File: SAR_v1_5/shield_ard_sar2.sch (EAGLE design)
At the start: 16 parts

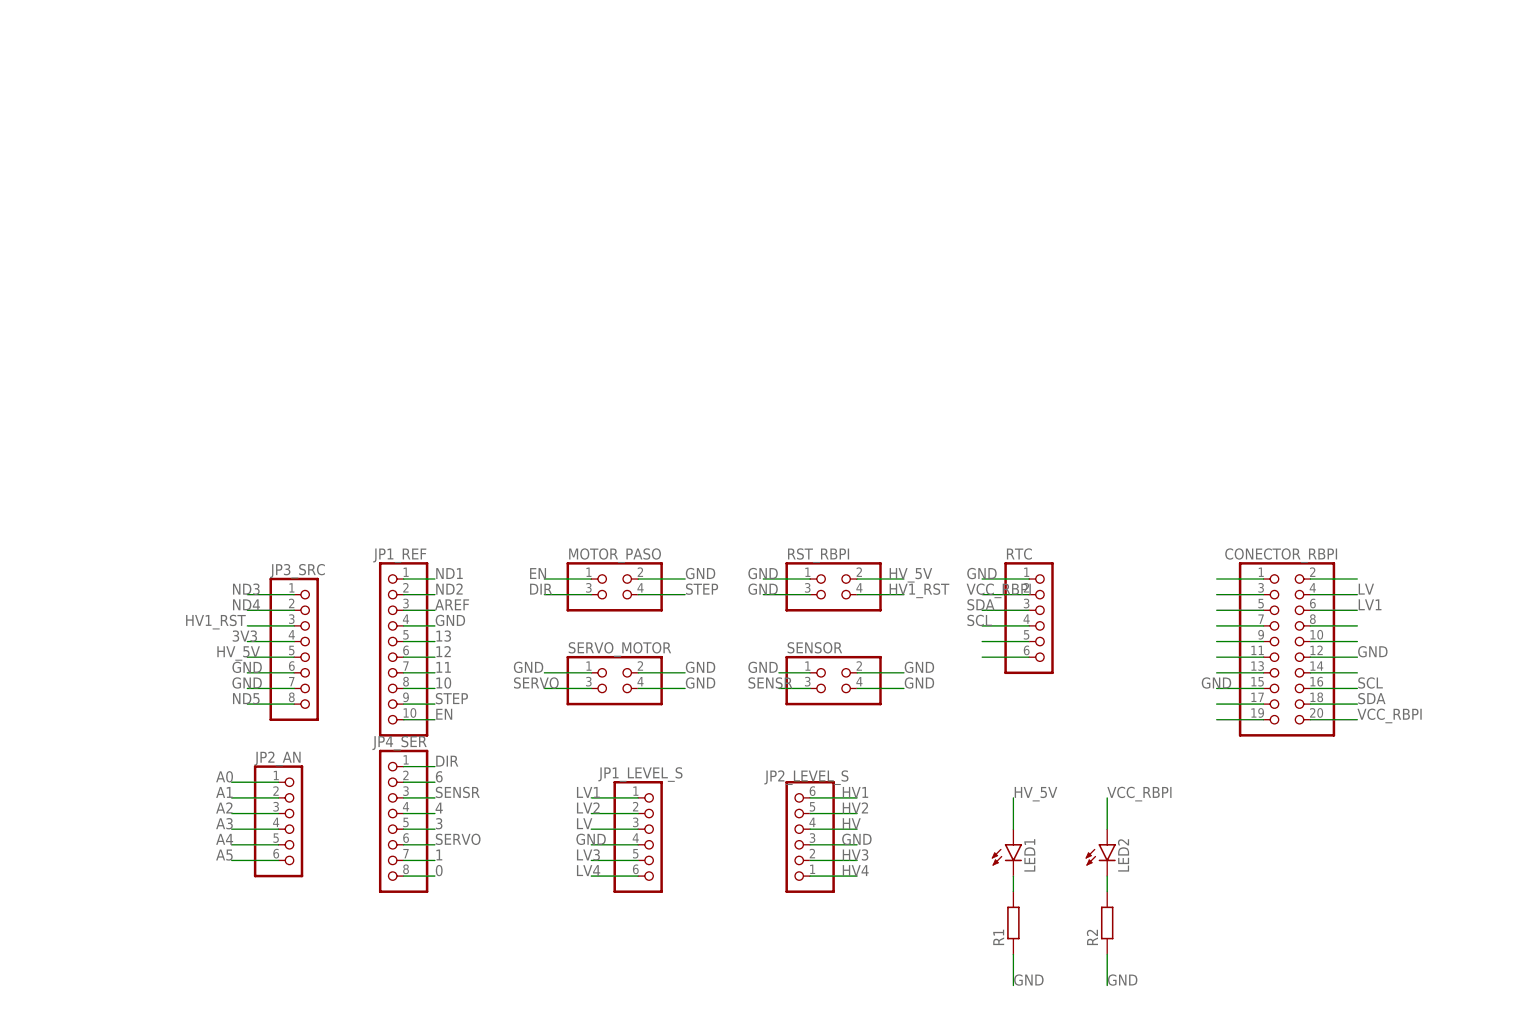
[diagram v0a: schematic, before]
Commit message: all the componentes were placed and routed correctly
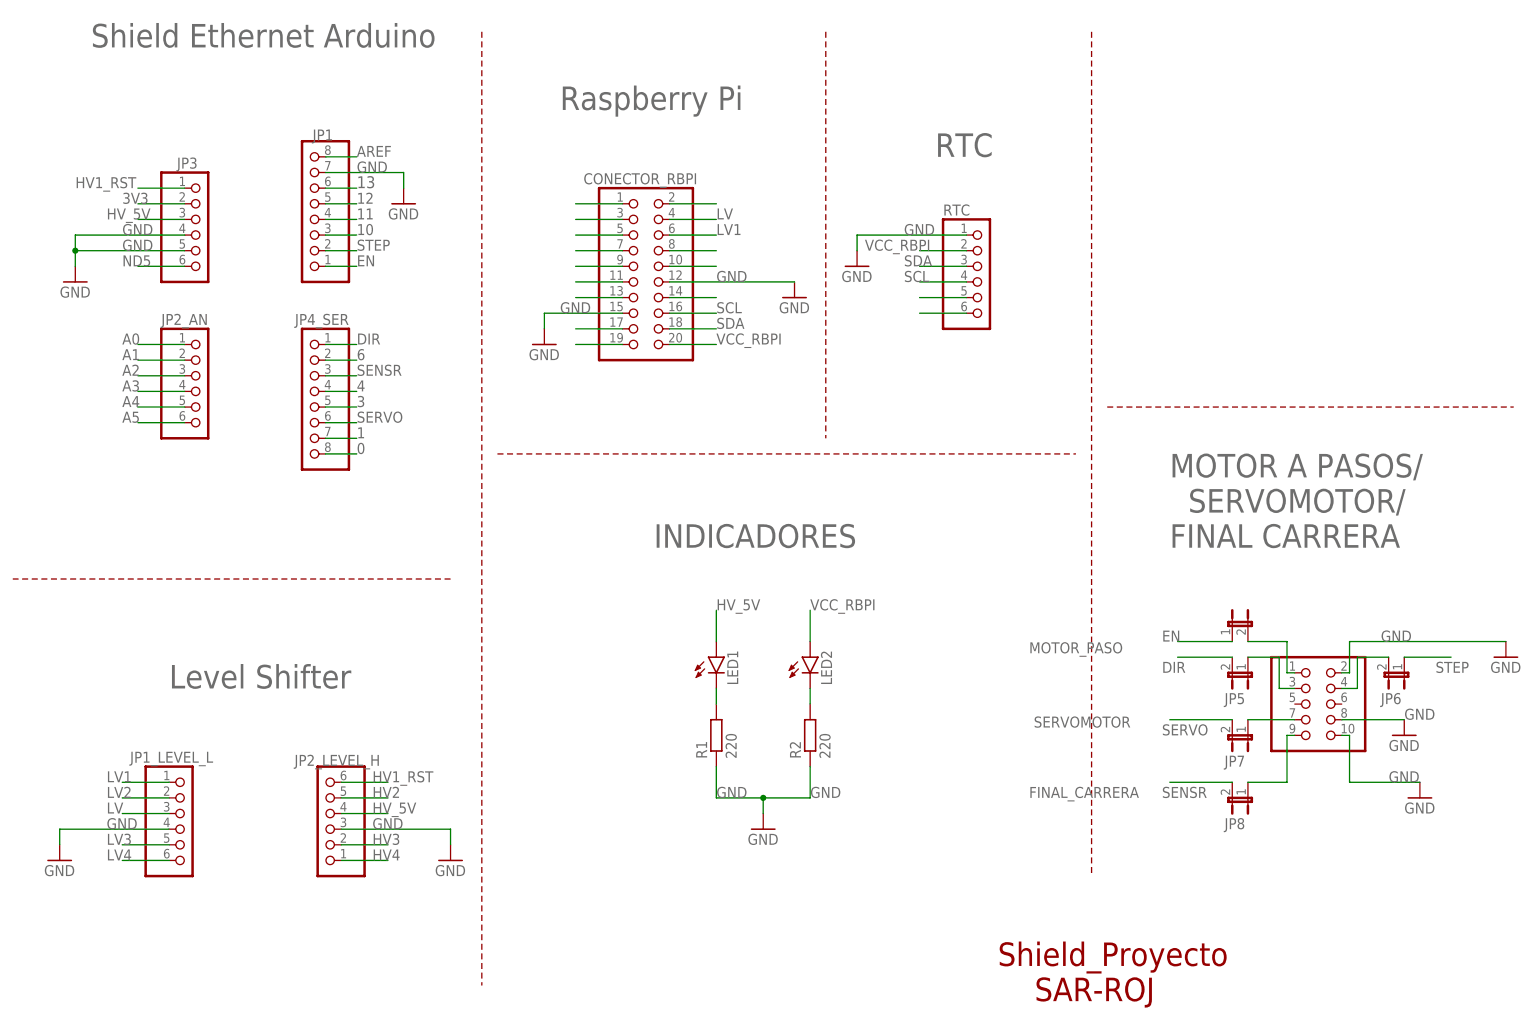
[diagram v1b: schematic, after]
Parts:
- removed JP1_LEVEL_S, JP2_LEVEL_S: (no value), pinhead:PINHD-1X6
- removed JP1_REF: (no value), pinhead:PINHD-1X10
- removed JP3_SRC: (no value), pinhead:PINHD-1X8
- removed RST_RBPI, SENSOR, SERVO_MOTOR: (no value), pinhead:PINHD-2X2
- added JP1: (no value), pinhead:PINHD-1X8
- added JP1_LEVEL_L, JP2_LEVEL_H, JP3: (no value), pinhead:PINHD-1X6
- added JP2, JP5, JP6, JP7, JP8: (no value), SparkFun-Retired:JUMPER-2PTH
- LED1, LED2: device led:LEDCHIP-LED0603 -> led:LEDCHIP-LED0805
- MOTOR_PASO: device pinhead:PINHD-2X2 -> pinhead:PINHD-2X5
- R1, R2: value (none) -> 220; device rcl:R-EU_R0603 -> rcl:R-EU_R0805
- RTC: device pinhead:PINHD-1X6 -> pinhead:PINHD-1X6/90
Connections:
- removed net HV: JP2_LEVEL_S.4
- removed net HV1: JP2_LEVEL_S.6
- removed net ND1: JP1_REF.1
- removed net ND2: JP1_REF.2
- removed net ND3: JP3_SRC.1
- removed net ND4: JP3_SRC.2
- new net DIR*: JP5.1, MOTOR_PASO.3
- new net EN*: JP2.2, MOTOR_PASO.1
- new net SENSR*: JP8.1, MOTOR_PASO.9
- new net SERVO*: JP7.1, MOTOR_PASO.7
- new net STEP*: JP6.2, MOTOR_PASO.4
- net 10: now also JP1.3; no longer JP1_REF.8
- net 11: now also JP1.4; no longer JP1_REF.7
- net 12: now also JP1.5; no longer JP1_REF.6
- net 13: now also JP1.6; no longer JP1_REF.5
- net 3V3: now also JP3.2; no longer JP3_SRC.4
- net AREF: now also JP1.8; no longer JP1_REF.3
- net DIR: now also JP5.2; no longer MOTOR_PASO.3
- net EN: now also JP1.1, JP2.1; no longer JP1_REF.10, MOTOR_PASO.1
- net GND: now also JP1.7, JP1_LEVEL_L.4, JP2_LEVEL_H.3, JP3.4, JP3.5, MOTOR_PASO.10, MOTOR_PASO.8; no longer JP1_LEVEL_S.4, JP1_REF.4, JP2_LEVEL_S.3, JP3_SRC.6, JP3_SRC.7, RST_RBPI.1, RST_RBPI.3, SENSOR.1, SENSOR.2, SENSOR.4, SERVO_MOTOR.1, SERVO_MOTOR.2, SERVO_MOTOR.4
- net HV1_RST: now also JP2_LEVEL_H.6, JP3.1; no longer JP3_SRC.3, RST_RBPI.4
- net HV2: now also JP2_LEVEL_H.5; no longer JP2_LEVEL_S.5
- net HV3: now also JP2_LEVEL_H.2; no longer JP2_LEVEL_S.2
- net HV4: now also JP2_LEVEL_H.1; no longer JP2_LEVEL_S.1
- net HV_5V: now also JP2_LEVEL_H.4, JP3.3; no longer JP3_SRC.5, RST_RBPI.2
- net LV: now also JP1_LEVEL_L.3; no longer JP1_LEVEL_S.3
- net LV1: now also JP1_LEVEL_L.1; no longer JP1_LEVEL_S.1
- net LV2: now also JP1_LEVEL_L.2; no longer JP1_LEVEL_S.2
- net LV3: now also JP1_LEVEL_L.5; no longer JP1_LEVEL_S.5
- net LV4: now also JP1_LEVEL_L.6; no longer JP1_LEVEL_S.6
- net ND5: now also JP3.6; no longer JP3_SRC.8
- net SENSR: now also JP8.2; no longer SENSOR.3
- net SERVO: now also JP7.2; no longer SERVO_MOTOR.3
- net STEP: now also JP1.2, JP6.1; no longer JP1_REF.9, MOTOR_PASO.4
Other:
- note added: "FINAL_CARRERA"
- note added: "INDICADORES"
- note added: "Level Shifter"
- note added: "MOTOR A PASOS/ SERVOMOTOR/ FINAL CARRERA"
- note added: "RTC"
- note added: "Raspberry Pi"
- note added: "SERVOMOTOR"
- note added: "Shield Ethernet Arduino"
- note added: "Shield_Proyecto SAR-ROJ"
- moved on the sheet: CONECTOR_RBPI, JP2_AN, JP4_SER, LED1, LED2, R1, R2, RTC
